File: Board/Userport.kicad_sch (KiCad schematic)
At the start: 31 parts, among them CN5 PORT_USER_PET_EDGE, U4 CD4053B, U5 CD4053B, X7 M09-182, X8 M09-182

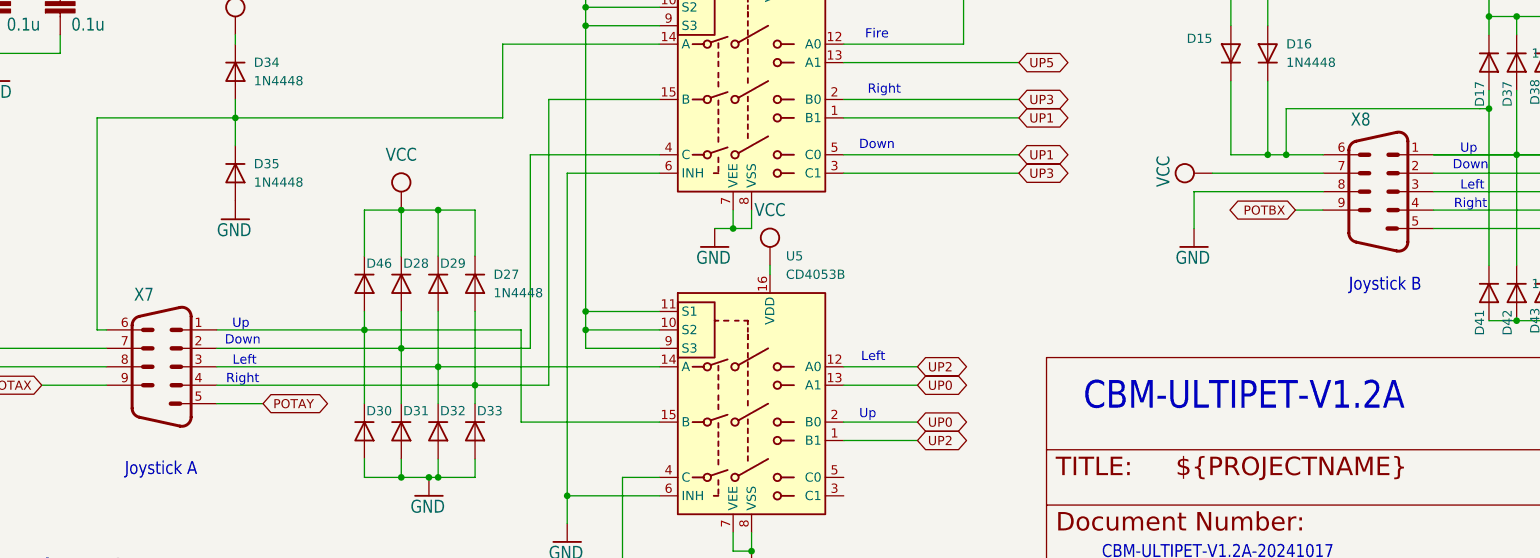
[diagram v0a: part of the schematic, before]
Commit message: work on 1.3
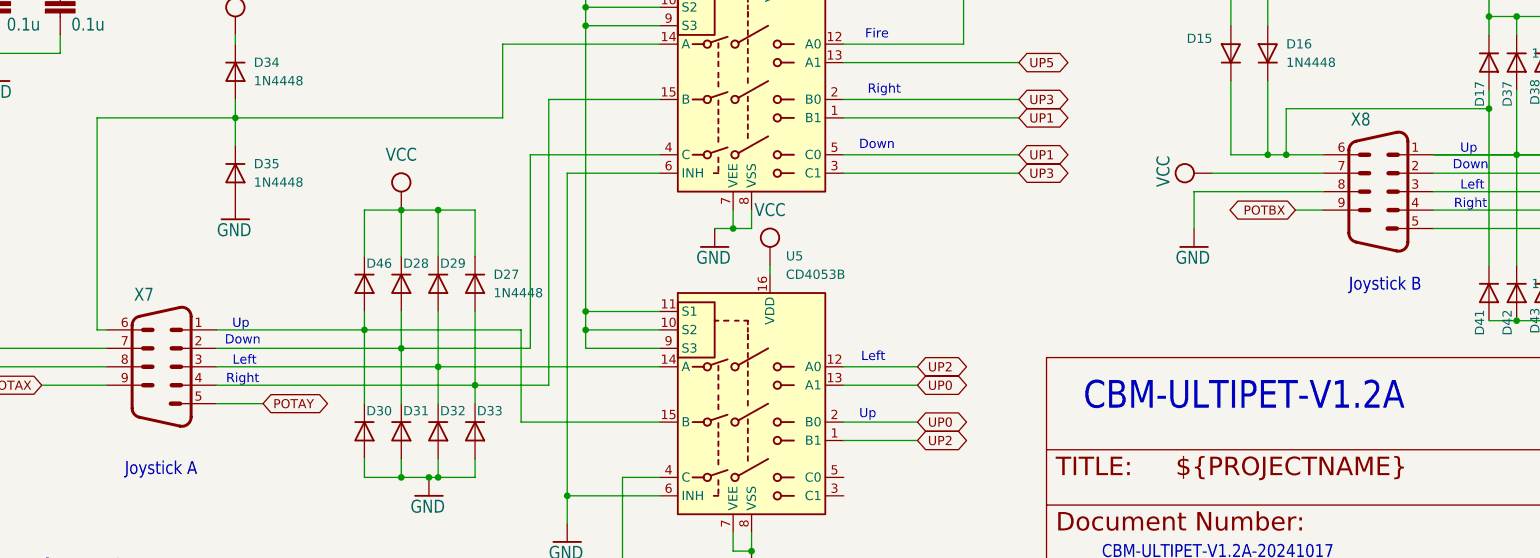
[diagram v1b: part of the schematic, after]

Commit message: work on r1.3
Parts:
- X7, X8: footprint cbm_ultipet_v1:182-009-MALE -> Connector_Dsub:DSUB-9_Pins_Horizontal_P2.77x2.84mm_EdgePinOffset9.90mm_Housed_MountingHolesOffset11.32mm
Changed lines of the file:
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@@
 			)
 		)
-		(property "Footprint" "cbm_ultipet_v1:182-009-MALE"
+		(property "Footprint" "Connector_Dsub:DSUB-9_Pins_Horizontal_P2.77x2.84mm_EdgePinOffset9.90mm_Housed_MountingHolesOffset11.32mm"
 			(at 60.96 153.67 0)
 			(effects
@@
 			)
 		)
-		(property "Footprint" "cbm_ultipet_v1:182-009-MALE"
+		(property "Footprint" "Connector_Dsub:DSUB-9_Pins_Horizontal_P2.77x2.84mm_EdgePinOffset9.90mm_Housed_MountingHolesOffset11.32mm"
 			(at 228.6 129.54 0)
 			(effects
